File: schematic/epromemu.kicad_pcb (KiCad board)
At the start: 2 copper layers, 82.3 x 54.1 mm, 10 parts, among them J1 EPROM Connector, U1 Teensy4.1, U2 74HC245, U3 74HC245, U4 74HC245, U5 74HC245

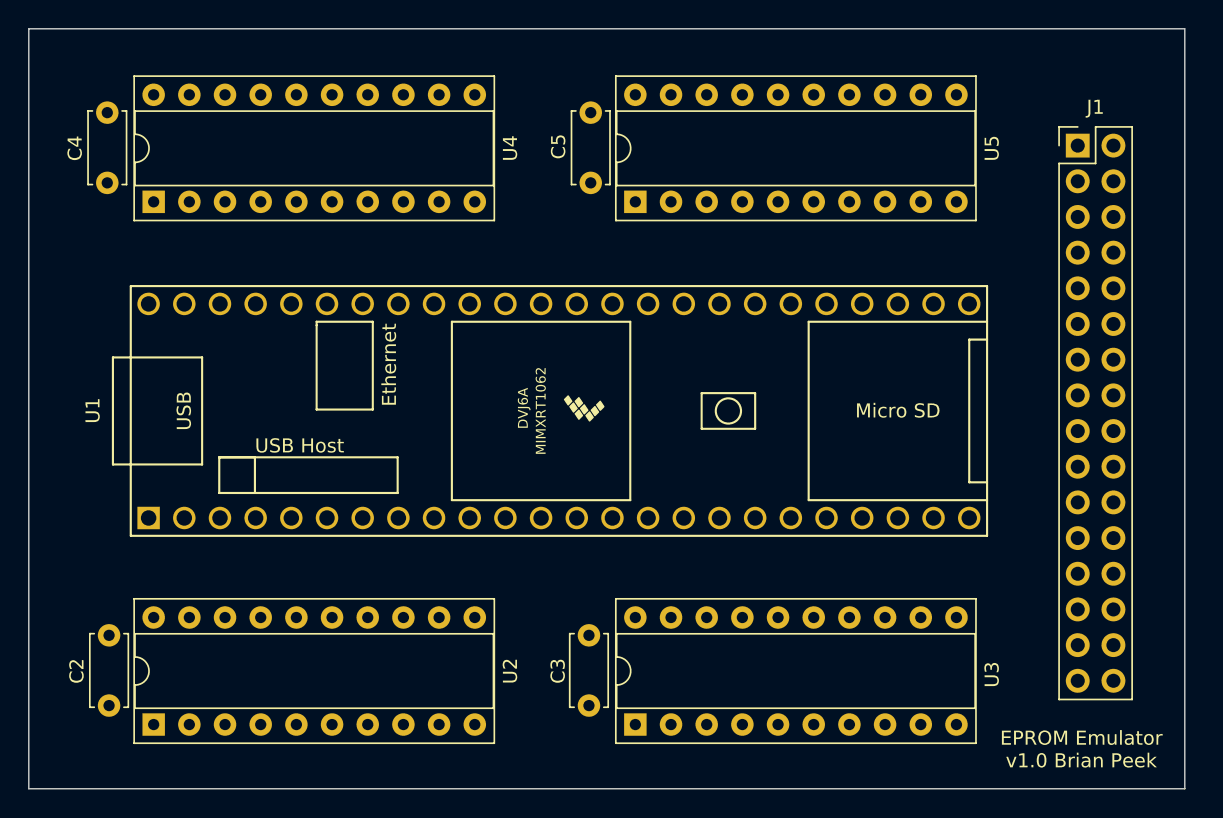
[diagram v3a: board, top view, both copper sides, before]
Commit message: final?
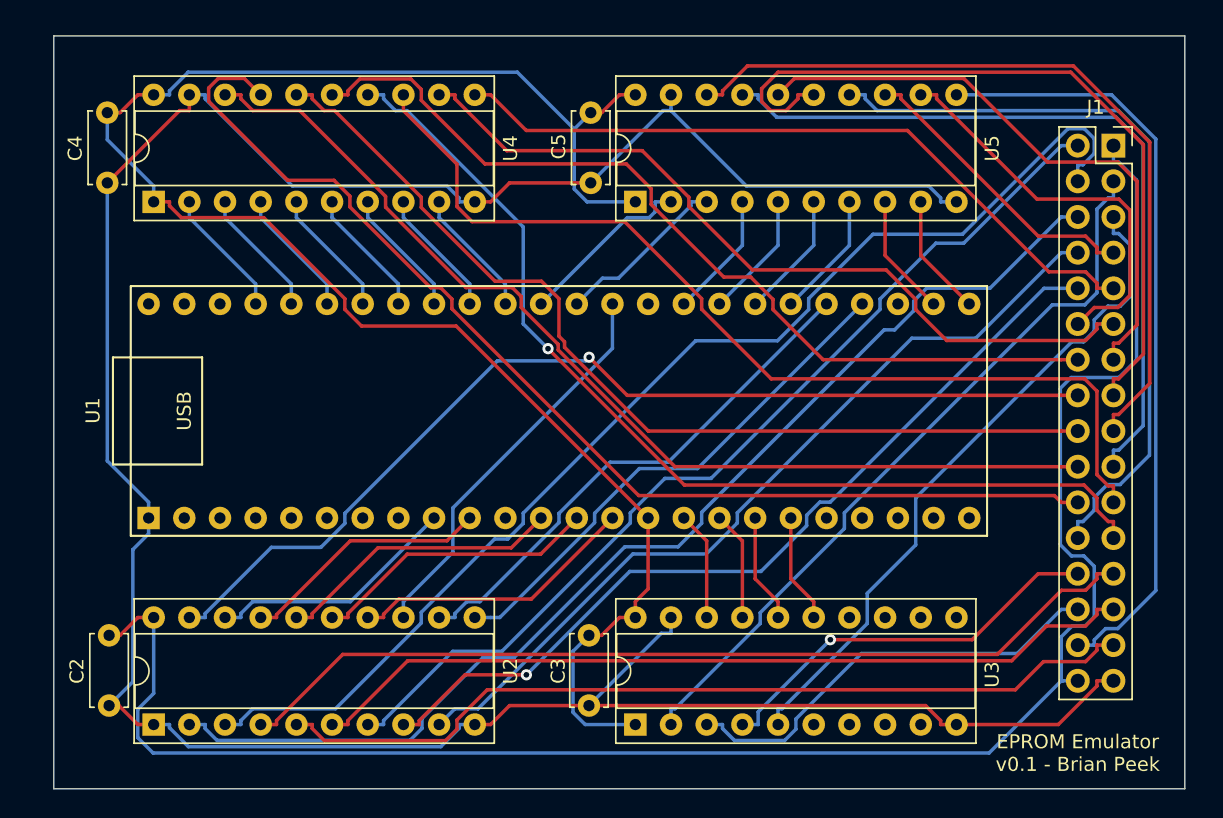
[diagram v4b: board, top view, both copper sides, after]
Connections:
- U1 pad 10: D7_3V3 -> D4_3V3
- U1 pad 11: D5_3V3 -> (no net)
- U1 pad 16: A0_3V3 -> A16_3V3
- U1 pad 17: A1_3V3 -> A17_3V3
- U1 pad 18: A16_3V3 -> A14_3V3
- U1 pad 19: A17_3V3 -> A15_3V3
- U1 pad 24: D6_3V3 -> (no net)
- U1 pad 28: (no net) -> D6_3V3
- U1 pad 29: (no net) -> D7_3V3
- U1 pad 30: A14_3V3 -> A12_3V3
- U1 pad 31: A15_3V3 -> A13_3V3
- U1 pad 32: A6_3V3 -> A4_3V3
- U1 pad 33: A7_3V3 -> A5_3V3
- U1 pad 36: A4_3V3 -> A2_3V3
- U1 pad 37: A5_3V3 -> A3_3V3
- U1 pad 38: A9_3V3 -> A7_3V3
- U1 pad 39: A8_3V3 -> A6_3V3
- U1 pad 40: A3_3V3 -> A1_3V3
- U1 pad 41: A2_3V3 -> A0_3V3
- U1 pad 42: A12_3V3 -> A10_3V3
- U1 pad 43: A13_3V3 -> A11_3V3
- U1 pad 44: A10_3V3 -> A8_3V3
- U1 pad 45: A11_3V3 -> A9_3V3
- U1 pad 8: D4_3V3 -> (no net)
- U1 pad 9: (no net) -> D5_3V3
- U2 pad 11: D3_3V3 -> D6_3V3
- U2 pad 12: D6_3V3 -> D7_3V3
- U2 pad 13: D1_3V3 -> D3_3V3
- U2 pad 14: D2_3V3 -> D1_3V3
- U2 pad 15: D0_3V3 -> D2_3V3
- U2 pad 16: D5_3V3 -> D0_3V3
- U2 pad 17: D7_3V3 -> D4_3V3
- U2 pad 18: D4_3V3 -> D5_3V3
- U2 pad 2: D4_5V -> D5_5V
- U2 pad 3: D7_5V -> D4_5V
- U2 pad 4: D5_5V -> D0_5V
- U2 pad 5: D0_5V -> D2_5V
- U2 pad 6: D2_5V -> D1_5V
- U2 pad 7: D1_5V -> D3_5V
- U2 pad 8: D6_5V -> D7_5V
- U2 pad 9: D3_5V -> D6_5V
- U3 pad 1: GND -> +3V3
- U3 pad 15: A17_3V3 -> A15_3V3
- U3 pad 16: A16_3V3 -> A14_3V3
- U3 pad 17: A1_3V3 -> A17_3V3
- U3 pad 18: A0_3V3 -> A16_3V3
- U3 pad 2: A0_5V -> A16_5V
- U3 pad 3: A1_5V -> A17_5V
- U3 pad 4: A16_5V -> A14_5V
- U3 pad 5: A17_5V -> A15_5V
- U4 pad 11: A9_5V -> A7_5V
- U4 pad 12: A8_5V -> A6_5V
- U4 pad 13: A3_5V -> A1_5V
- U4 pad 14: A2_5V -> A0_5V
- U4 pad 15: A12_5V -> A10_5V
- U4 pad 16: A13_5V -> A11_5V
- U4 pad 17: A10_5V -> A8_5V
- U4 pad 18: A11_5V -> A9_5V
- U4 pad 2: A11_3V3 -> A9_3V3
- U4 pad 3: A10_3V3 -> A8_3V3
- U4 pad 4: A13_3V3 -> A11_3V3
- U4 pad 5: A12_3V3 -> A10_3V3
- U4 pad 6: A2_3V3 -> A0_3V3
- U4 pad 7: A3_3V3 -> A1_3V3
- U4 pad 8: A8_3V3 -> A6_3V3
- U4 pad 9: A9_3V3 -> A7_3V3
- U5 pad 13: A15_5V -> A12_5V
- U5 pad 14: A14_5V -> A13_5V
- U5 pad 15: A6_5V -> A4_5V
- U5 pad 16: A7_5V -> A5_5V
- U5 pad 17: A4_5V -> A2_5V
- U5 pad 18: A5_5V -> A3_5V
- U5 pad 2: A5_3V3 -> A3_3V3
- U5 pad 3: A4_3V3 -> A2_3V3
- U5 pad 4: A7_3V3 -> A5_3V3
- U5 pad 5: A6_3V3 -> A4_3V3
- U5 pad 6: A15_3V3 -> A13_3V3
- U5 pad 7: A14_3V3 -> A12_3V3
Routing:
- net GND: track 0.00 -> 199.0 mm
- net +5V: track 0.00 -> 128.5 mm
- net +3V3: track 0.00 -> 125.5 mm
- net D4_5V: track 0.00 -> 85.0 mm
- net D5_5V: track 0.00 -> 80.6 mm
- net A8_5V: track 0.00 -> 80.0 mm
- net A9_5V: track 0.00 -> 73.0 mm
- net OE_5V: track 0.00 -> 72.6 mm, vias 0 -> 1
- net A0_5V: track 0.00 -> 71.6 mm, vias 0 -> 1
- net A1_5V: track 0.00 -> 69.6 mm
- net D3_5V: track 0.00 -> 68.6 mm
- net A11_5V: track 0.00 -> 67.9 mm
- net D0_5V: track 0.00 -> 65.5 mm
- net A10_5V: track 0.00 -> 63.5 mm
- net D2_5V: track 0.00 -> 62.2 mm
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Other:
- board size 82.3 x 54.1 mm -> 80.5 x 53.6 mm
- net class Default: clearance 0.2 -> 0.1524; trace_width 0.25 -> 0.1524; via_dia 0.8 -> 0.6858; via_drill 0.4 -> 0.3302
- rule pad_to_mask_clearance: 0 -> 0.0508
- rule trace_clearance: 0.2 -> 0.1524
- rule trace_min: 0.2 -> 0.1524
- rule via_min_drill: 0.3 -> 0.254
- rule via_min_size: 0.4 -> 0.508
- board text added: "EPROM Emulator v0.1 - Brian Peek"
- board text removed: "EPROM Emulator v1.0 Brian Peek"

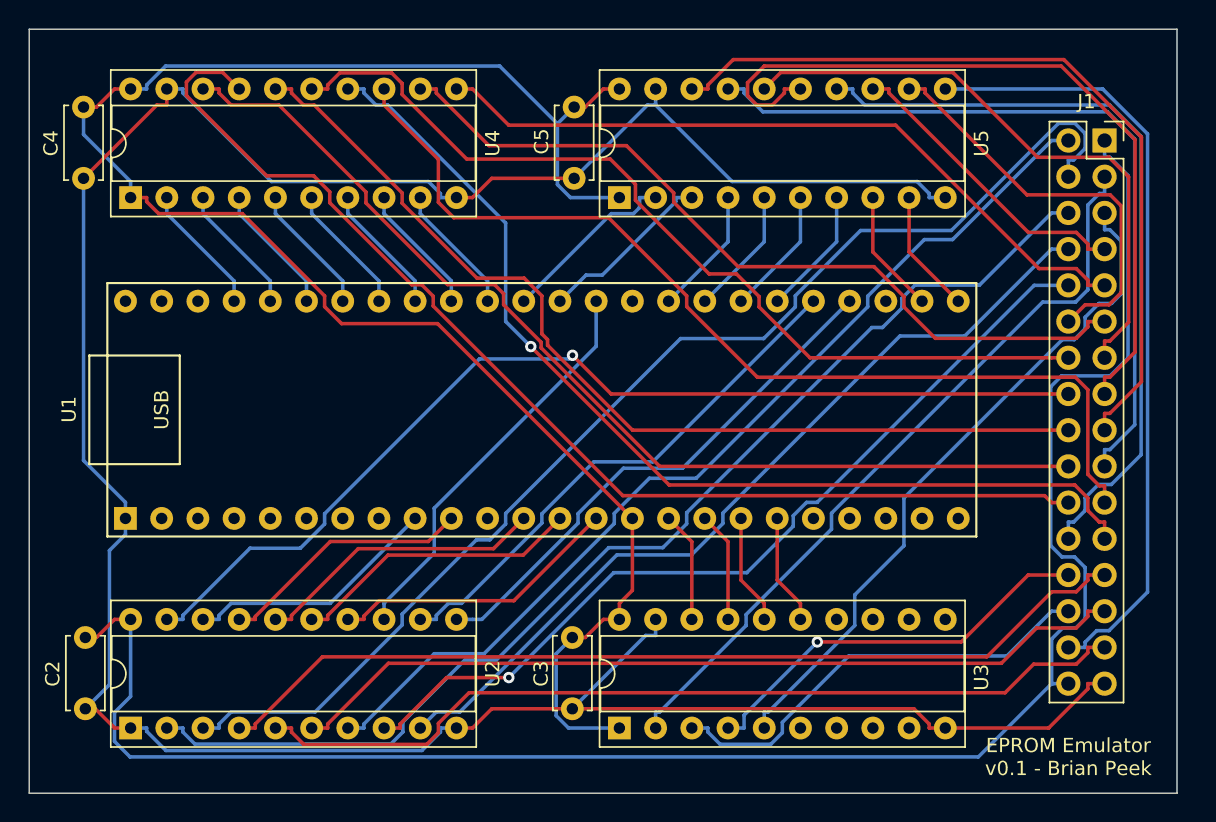
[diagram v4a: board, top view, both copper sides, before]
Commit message: submitted v0.1
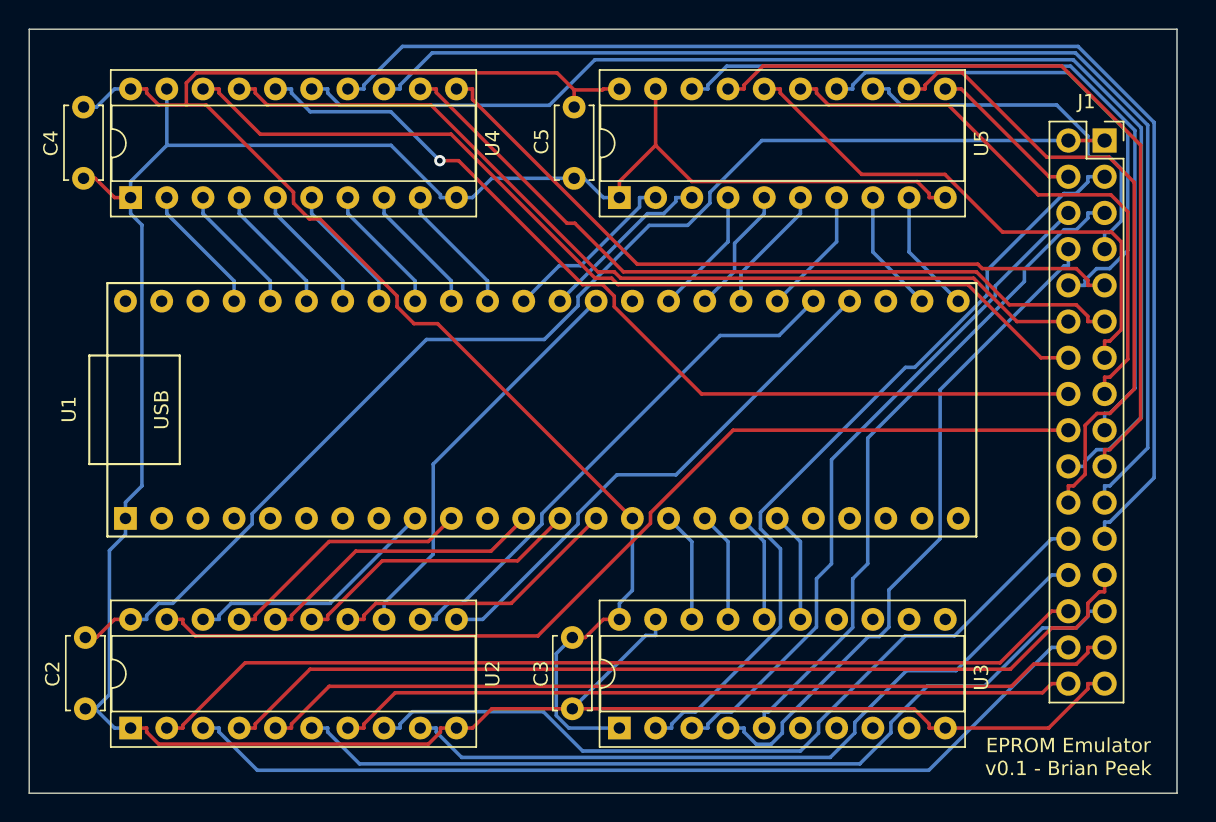
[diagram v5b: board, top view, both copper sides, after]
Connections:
- U4 pad 1: +3V3 -> GND
- U5 pad 1: +3V3 -> GND
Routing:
- net PGM_5V: track 55.0 -> 11.2 mm
- net +5V: track 128.5 -> 87.3 mm
- net A10_5V: track 63.5 -> 89.2 mm
- net A0_5V: track 71.6 -> 91.0 mm, vias 1 -> 0
- net D4_5V: track 85.0 -> 65.7 mm
- net A14_5V: track 28.8 -> 47.7 mm, vias 1 -> 0
- net A13_5V: track 54.0 -> 36.5 mm
- net +3V3: track 125.5 -> 108.5 mm
- net A17_5V: track 31.3 -> 48.2 mm
- net D3_5V: track 68.6 -> 52.0 mm
- net CE_5V: track 29.1 -> 44.7 mm
- net A1_5V: track 69.6 -> 84.8 mm
- net A8_5V: track 80.0 -> 65.1 mm
- net A4_5V: track 54.3 -> 40.4 mm
- net D5_5V: track 80.6 -> 66.8 mm
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
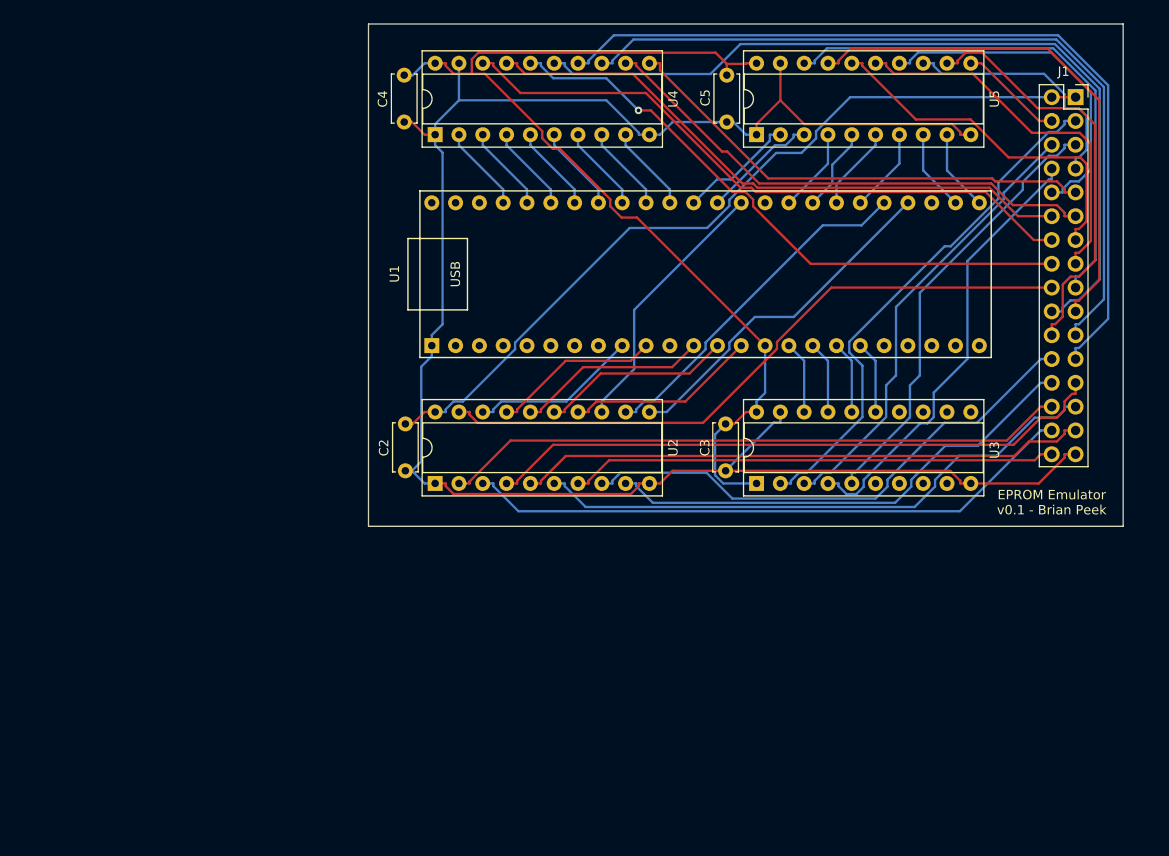
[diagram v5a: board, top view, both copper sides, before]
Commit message: update to v6
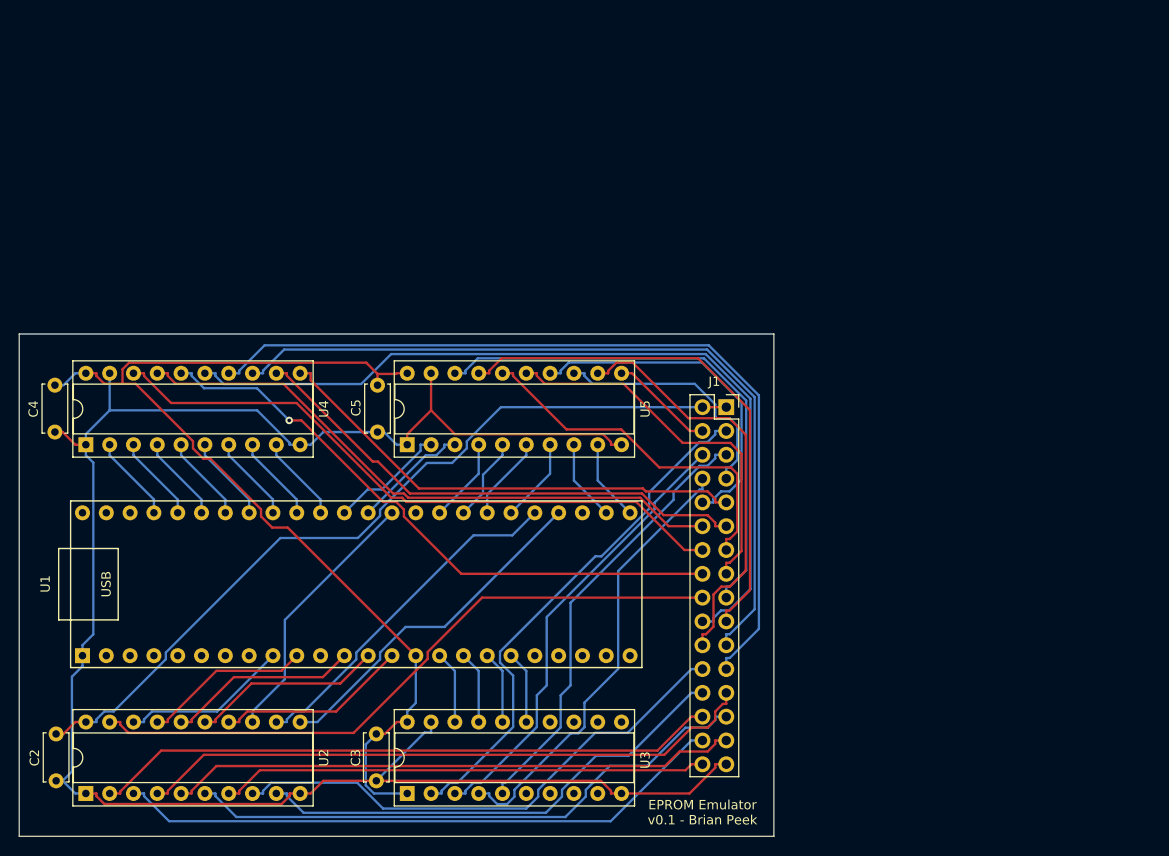
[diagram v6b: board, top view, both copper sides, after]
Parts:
- moved U4 49.8 mm to (112.6, 82.5)
- moved C2 49.8 mm to (109.4, 113.3)
- moved C3 49.8 mm to (143.6, 113.3)
- moved C4 49.8 mm to (109.3, 76.1)
- moved C5 49.8 mm to (143.7, 76.1)
- moved J1 49.8 mm to (178.4, 78.5)
- moved U2 49.8 mm to (112.6, 119.7)
- moved U5 49.8 mm to (146.9, 82.5)
- moved U1 49.8 mm to (141.4, 97.4)
- moved U3 49.8 mm to (146.9, 119.7)
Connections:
- U1 pad 11: (no net) -> unconnected-(U1-Pad11)
- U1 pad 2: (no net) -> unconnected-(U1-Pad2)
- U1 pad 20: (no net) -> unconnected-(U1-Pad20)
- U1 pad 21: (no net) -> unconnected-(U1-Pad21)
- U1 pad 22: (no net) -> unconnected-(U1-Pad22)
- U1 pad 23: (no net) -> unconnected-(U1-Pad23)
- U1 pad 24: (no net) -> unconnected-(U1-Pad24)
- U1 pad 27: (no net) -> unconnected-(U1-Pad27)
- U1 pad 3: (no net) -> unconnected-(U1-Pad3)
- U1 pad 34: (no net) -> unconnected-(U1-Pad34)
- U1 pad 4: (no net) -> unconnected-(U1-Pad4)
- U1 pad 46: (no net) -> unconnected-(U1-Pad46)
- U1 pad 47: (no net) -> unconnected-(U1-Pad47)
- U1 pad 48: (no net) -> unconnected-(U1-Pad48)
- U1 pad 5: (no net) -> unconnected-(U1-Pad5)
- U1 pad 6: (no net) -> unconnected-(U1-Pad6)
- U1 pad 7: (no net) -> unconnected-(U1-Pad7)
- U1 pad 8: (no net) -> unconnected-(U1-Pad8)
- U3 pad 11: (no net) -> unconnected-(U3-Pad11)
- U3 pad 12: (no net) -> unconnected-(U3-Pad12)
- U3 pad 13: (no net) -> unconnected-(U3-Pad13)
- U3 pad 14: (no net) -> unconnected-(U3-Pad14)
- U3 pad 6: (no net) -> unconnected-(U3-Pad6)
- U3 pad 7: (no net) -> unconnected-(U3-Pad7)
- U3 pad 8: (no net) -> unconnected-(U3-Pad8)
- U3 pad 9: (no net) -> unconnected-(U3-Pad9)
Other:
- net class Default removed
